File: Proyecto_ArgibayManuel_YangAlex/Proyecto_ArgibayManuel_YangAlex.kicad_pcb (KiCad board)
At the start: 2 copper layers, 159 x 89.5 mm, 61 parts, among them IC1 LM1117, J1 Conn_01x02, J2 Conn_01x01, J3 Con_1x2, J4 Con_1x3, J5 Conn_01x03_Pin, J6 Conn_01x07, J7 Con_ICSP, K1 RT314012, K2 RT314012, Q1 2N2222, Q2 2N2222, SW1 SW_Push, SW2 SW_Push, SW3 SW_Push, SW4 SW_Push, U1 PIC18F258-I_SO, U2 HDC2010YPAR, U3 LT1716IS5TRMPBF, U4 LT1716IS5TRMPBF, U5 TXS0108EPW, U6 DRV8871DDA, U7 DRV8871DDA, U8 MCP2551-I-P, X1 DB9, X2 DB9, Y1 Crystal

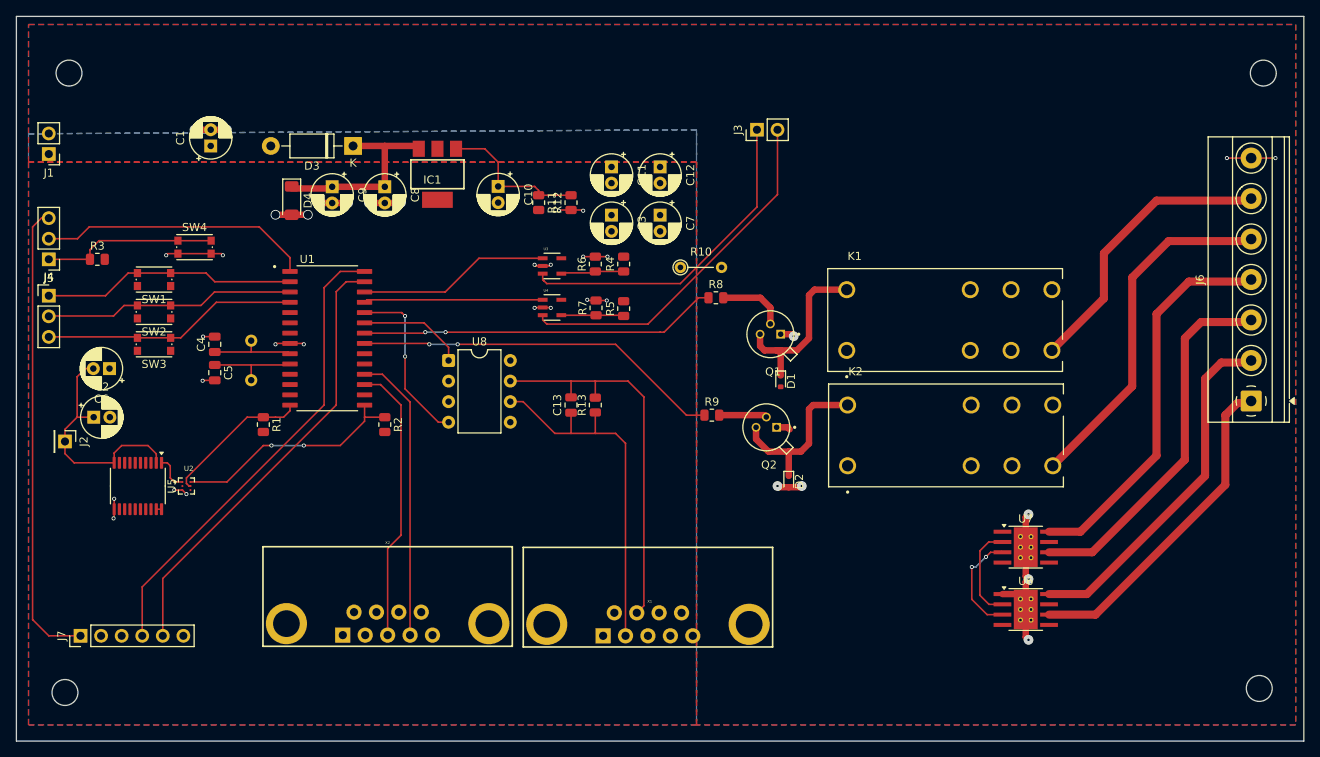
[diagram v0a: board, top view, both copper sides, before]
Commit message: Agrego cambios
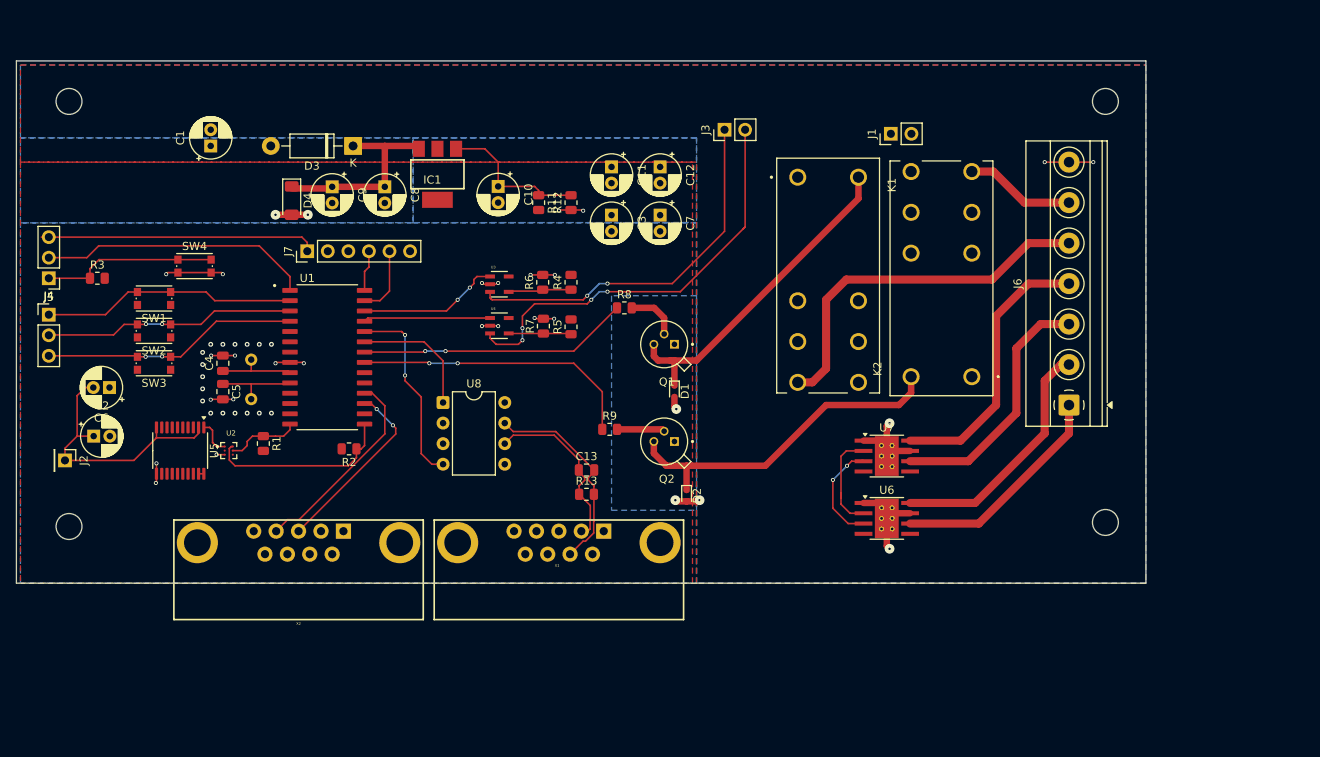
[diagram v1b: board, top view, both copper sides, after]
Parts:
- removed R10: 0, Resistor_THT:R_Axial_DIN0204_L3.6mm_D1.6mm_P5.08mm_Vertical
- moved J1 104.0 mm to (204.0, 41.0), turned to 90 degrees
- moved J7 55.1 mm to (131.9, 55.5)
- moved REF** 28.0 mm to (230.5, 89.0)
- moved J6 22.5 mm to (226.0, 74.5)
- moved U6 20.5 mm to (203.5, 88.5)
- moved U7 20.5 mm to (203.5, 80.8)
- moved Ref 20.5 mm to (102.5, 89.5)
- moved REF** 19.8 mm to (230.5, 37.0)
- moved K2 19.4 mm to (210.2, 58.9), turned to 90 degrees
- moved K1 15.5 mm to (196.2, 58.5), turned to -90 degrees
- moved X1 14.9 mm to (163.0, 91.5), turned to 180 degrees
- moved X2 14.9 mm to (130.8, 91.5), turned to 180 degrees
- moved Q1 13.2 mm to (176.0, 67.0)
- moved D1 13.2 mm to (177.3, 72.8)
- moved Q2 12.7 mm to (176.0, 79.0)
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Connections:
- net CANH renamed CAN+
- net CANL renamed CAN-
- J1 pad 1: GND -> GNDPWR
- J6 pad 5: Calefactor -> Bomba
- J6 pad 6: Bomba -> Calefactor
- J6 pad 7: GND -> GNDPWR
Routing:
- net PGD: track 58.1 -> 5.06 mm
- net PGC: track 55.4 -> 8.49 mm
- net Calefactor: track 43.7 -> 13.6 mm
- net CAN-: track 45.3 -> 21.7 mm
- net VPP: track 57.7 -> 34.2 mm
- net CAN+: track 48.4 -> 25.8 mm
- net Net-(D2-K): track 21.3 -> 42.6 mm
- net Net-(D1-K): track 21.7 -> 41.0 mm
- net Motor_derecho_2: track 45.3 -> 31.3 mm
- net Motor_derecho_1: track 47.8 -> 34.1 mm
- net Motor_Izquierdo_1: track 43.6 -> 30.5 mm
- net Motor_izquierdo_2: track 40.6 -> 27.7 mm
- net RC6: track 34.6 -> 22.8 mm, vias 0 -> 2
- net C_R_Bombas_agua: track 44.3 -> 33.4 mm
- net RC7: track 35.8 -> 25.0 mm
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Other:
- board size 159 x 89.5 mm -> 139.5 x 64.5 mm

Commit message: Arreglo layout y esqumatico con las correcciones pasadas
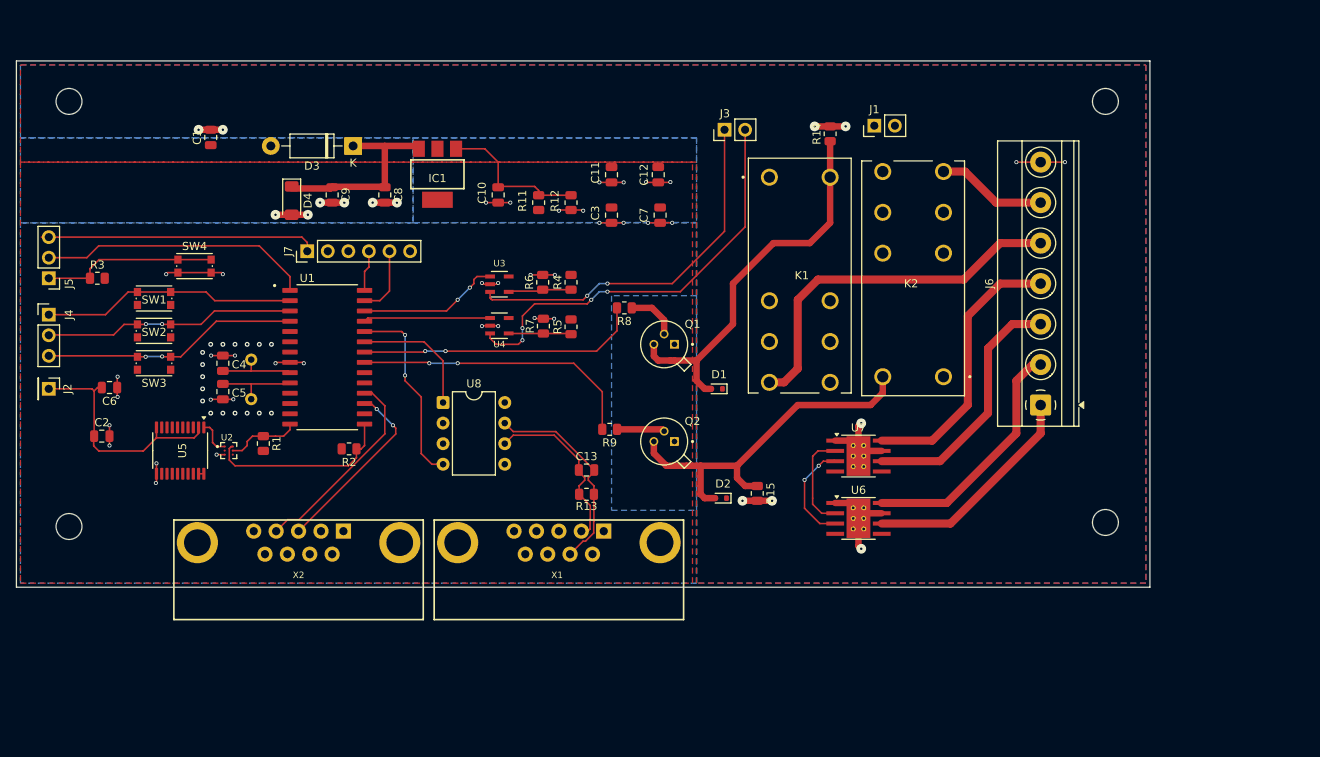
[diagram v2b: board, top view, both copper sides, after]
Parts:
- added R14: 1k, Resistor_SMD:R_0805_2012Metric, F.Cu at (196.5, 41.0)
- added R15: 1k, Resistor_SMD:R_0805_2012Metric, F.Cu at (187.5, 85.4)
- C1, C10, C11, C12, C2, C3, C6, C7, C8, C9: footprint Capacitor_THT:CP_Radial_D5.0mm_P2.00mm -> Capacitor_SMD:C_0805_2012Metric
- moved J2 9.06 mm to (100.0, 72.5)
- moved D1 5.24 mm to (182.5, 72.5), turned to 180 degrees
- moved D2 4.24 mm to (183.0, 86.0), turned to 180 degrees
- moved J6 3.50 mm to (222.5, 74.5)
- moved K1 3.50 mm to (192.8, 58.5)
- moved K2 3.50 mm to (206.8, 58.9)
- moved U6 3.50 mm to (200.0, 88.5)
- moved U7 3.50 mm to (200.0, 80.8)
- moved J1 2.27 mm to (202.0, 40.0)
- moved C1 1.05 mm to (120.0, 41.5)
- moved C10 1.05 mm to (155.5, 48.5)
- moved C2 1.01 mm to (106.5, 78.3)
- moved C8 1.01 mm to (141.5, 48.5)
- moved C9 1.01 mm to (135.0, 48.5)
- moved C12 0.99 mm to (175.3, 46.0)
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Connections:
- D1 pad 1: Net-(D1-K) -> VBat
- D1 pad 2: GNDPWR -> Net-(D1-A)
- D2 pad 1: Net-(D2-K) -> VBat
- D2 pad 2: GNDPWR -> Net-(D2-A)
- K1 pad A2: Net-(D1-K) -> Net-(D1-A)
- K2 pad A2: Net-(D2-K) -> Net-(D2-A)
- Q1 pad 3: Net-(D1-K) -> Net-(D1-A)
- Q2 pad 3: Net-(D2-K) -> Net-(D2-A)
- R8 pad 1: C_R_Bombas_agua -> Net-(Q1-Pad2)
- R8 pad 2: Net-(Q1-Pad2) -> C_R_Bombas_agua
- R9 pad 1: C_R_Calefactor -> Net-(Q2-Pad2)
- R9 pad 2: Net-(Q2-Pad2) -> C_R_Calefactor
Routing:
- net Net-(D1-A): track 0.00 -> 48.2 mm
- net Net-(D2-A): track 0.00 -> 46.0 mm
- net Net-(D2-K): track 42.6 -> 0.00 mm
- net Net-(D1-K): track 41.0 -> 0.00 mm
- net GND: track 32.8 -> 52.9 mm, vias 21 -> 35
- net GNDPWR: track 35.8 -> 47.8 mm, vias 9 -> 16
- net +3.3V: track 33.0 -> 29.8 mm
- net C_R_Bombas_agua: track 33.4 -> 35.1 mm
- net PH_M_in2: track 12.9 -> 12.2 mm
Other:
- board size 139.5 x 64.5 mm -> 140 x 65 mm
